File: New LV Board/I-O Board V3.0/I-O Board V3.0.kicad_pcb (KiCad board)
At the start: 2 copper layers, 58.1 x 146.2 mm, 22 parts, among them J1 PH1-10-UA, J10 691137710002, J11 691137710002, J12 20-0600-21, J12 Conn_01x15, J13 Conn_01x15, J2 *, J3 *, J4 *, J5 Conn_01x15, J6 20-0600-21, J7 691137710002, J8 691137710002, J9 691137710002

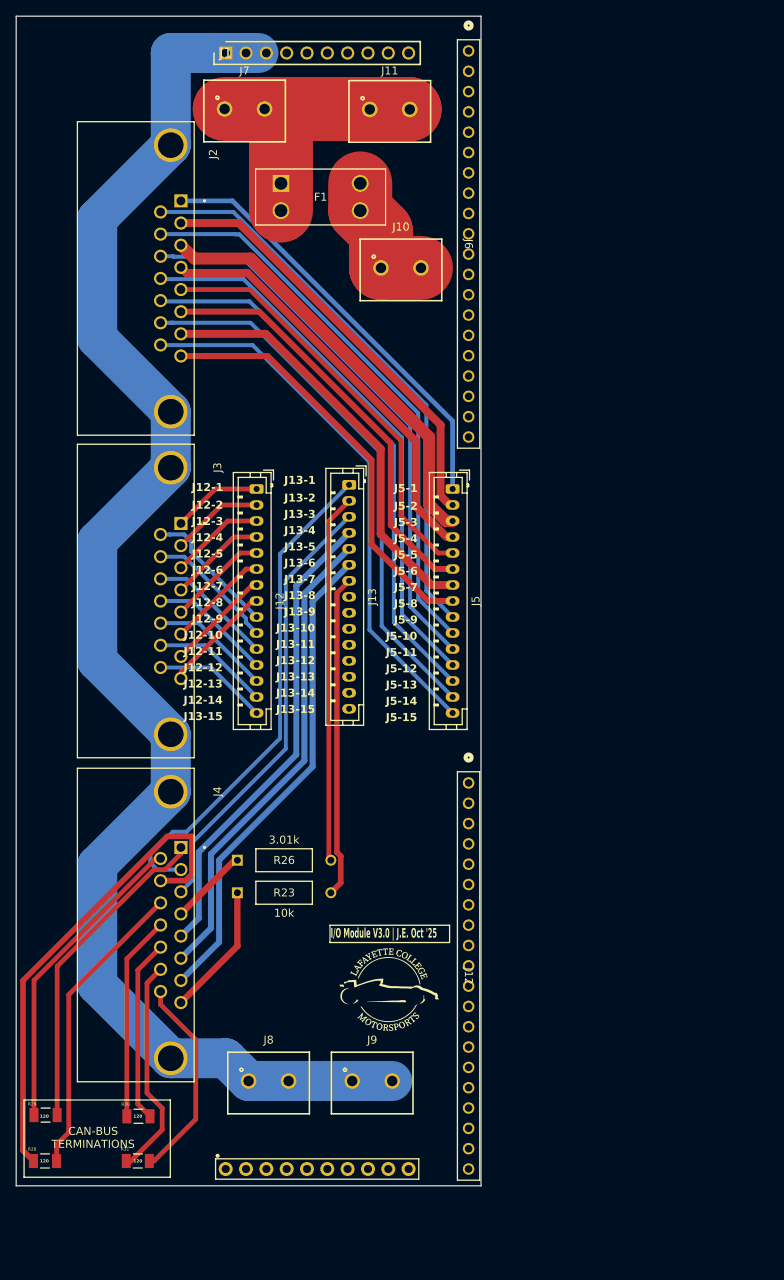
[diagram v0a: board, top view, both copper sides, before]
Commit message: IO Board V3.0 done?
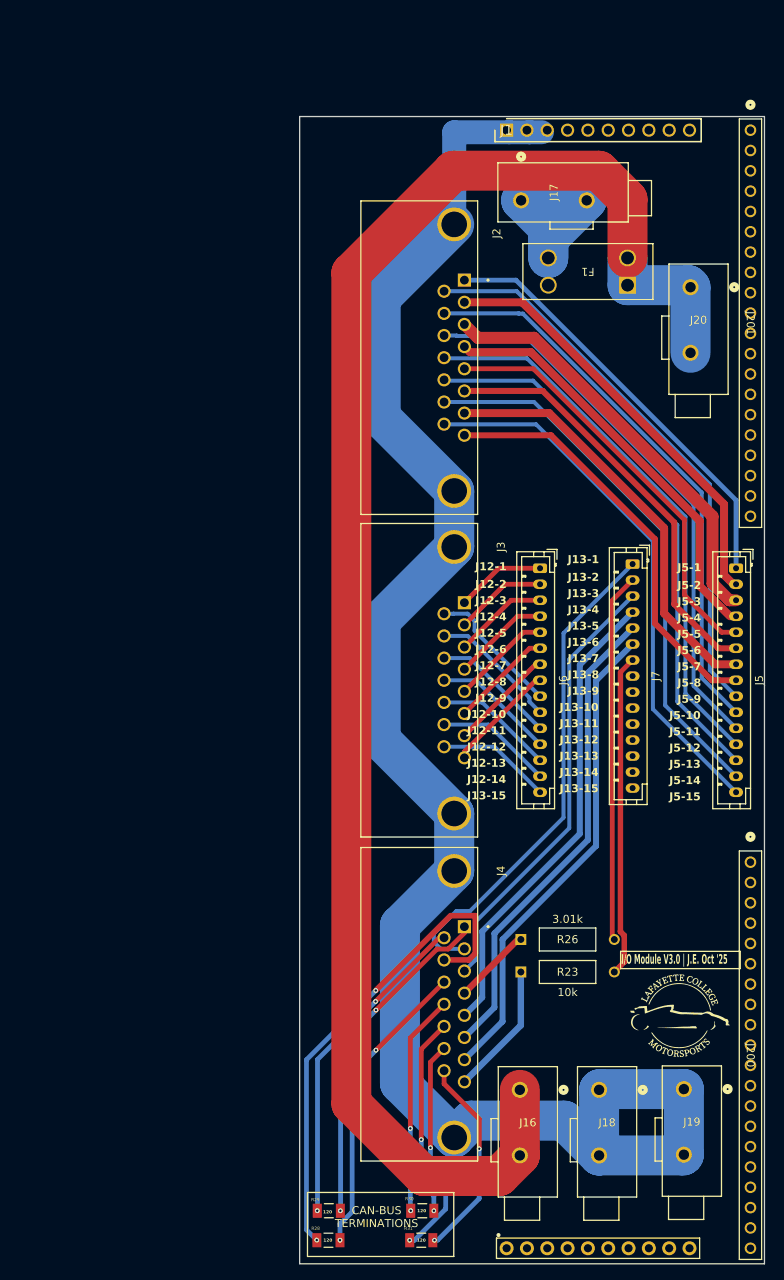
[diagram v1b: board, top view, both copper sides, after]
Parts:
- removed J10, J11, J8, J9: 691137710002, I-O_Footprints:691137710002
- removed the J7 at (86.5, 27.0)
- added J16: 2604-1101, MotorSports_KICad:CONN_2604-1101_WAG, F.Cu at (120.9, 149.6)
- added J17: 2604-1101, MotorSports_KICad:CONN_2604-1101_WAG, F.Cu at (121.1, 38.4)
- added J18: 2604-1101, MotorSports_KICad:CONN_2604-1101_WAG, F.Cu at (130.8, 149.6)
- added J19: 2604-1101, MotorSports_KICad:CONN_2604-1101_WAG, F.Cu at (141.4, 149.5)
- added J20: 2604-1101, MotorSports_KICad:CONN_2604-1101_WAG, F.Cu at (142.2, 49.3)
- moved F1 45.1 mm to (134.4, 49.0), turned to 180 degrees
- moved R30 37.4 mm to (108.7, 164.7)
- moved R29 37.4 mm to (97.0, 164.7)
- moved J2 36.8 mm to (112.7, 58.1)
- moved J3 36.8 mm to (112.7, 98.4)
- moved J4 36.8 mm to (112.7, 138.9)
- moved J6 36.8 mm to (123.4, 84.4)
- moved J7 36.8 mm to (135.0, 83.9)
- moved R23 36.8 mm to (121.0, 134.9)
- moved R26 36.8 mm to (121.0, 130.8)
- moved R28 36.8 mm to (97.0, 168.4)
- moved J5 36.8 mm to (147.9, 84.4)
- moved R31 36.8 mm to (108.6, 168.4)
- moved J200 36.6 mm to (149.7, 121.1)
- moved J201 36.6 mm to (149.7, 29.6)
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- renumbered J12 to J200, J6 to J201, J12 to J6, J13 to J7
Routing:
- net Net-(J16-1_1): track 33.8 -> 206.1 mm
- net Net-(J18-1_1): track 188.3 -> 215.9 mm
- net Net-(J17-1_1): track 16.6 -> 26.0 mm
- net Net-(J4-Pad01): track 40.7 -> 42.8 mm, vias 0 -> 2
- net Net-(J4-Pad09): track 39.0 -> 41.0 mm, vias 0 -> 2
- net Net-(J4-Pad13): track 22.9 -> 24.9 mm, vias 0 -> 2
- net Net-(J4-Pad12): track 25.7 -> 27.6 mm, vias 0 -> 2
- net Net-(J4-Pad10): vias 0 -> 2
- net Net-(J4-Pad15): vias 0 -> 2
- net Net-(J4-Pad14): vias 0 -> 2
- net Net-(J4-Pad11): vias 0 -> 2
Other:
- board size 58.1 x 146.2 mm -> 58.1 x 143.4 mm
